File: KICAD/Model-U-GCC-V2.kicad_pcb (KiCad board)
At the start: 2 copper layers, 28.5 x 13 mm, 7 parts, among them J1 USB_C_Receptacle, J2 Conn_01x06, J3 Conn_01x02

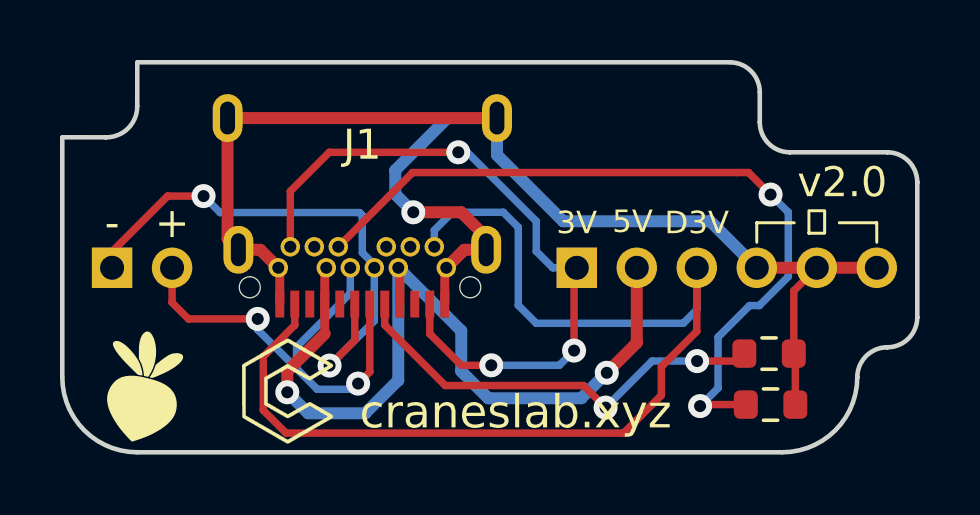
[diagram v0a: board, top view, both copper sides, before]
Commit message: 00000
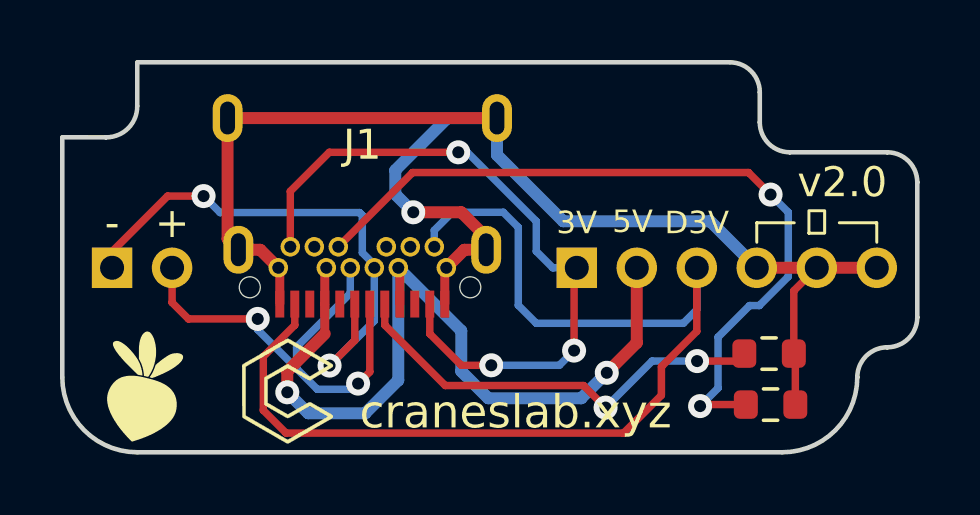
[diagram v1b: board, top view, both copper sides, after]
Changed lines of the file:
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@@
   (via (at 129.3041 107.5941) (size 0.8) (drill 0.4) (layers "F.Cu" "B.Cu") (net 5))
   (segment (start 132.65 109.75) (end 132.46 109.94) (width 0.25) (layer "B.Cu") (net 5))
-  (segment (start 130.6 108.89) (end 130.6 108.53) (width 0.25) (layer "B.Cu") (net 5))
+  (segment (start 130.6 109.25) (end 130.6 108.53) (width 0.25) (layer "B.Cu") (net 5))
   (segment (start 129.3041 107.9541) (end 129.3041 107.5941) (width 0.25) (layer "B.Cu") (net 5))
   (segment (start 132.39 106.74) (end 132.39 105.89) (width 0.25) (layer "B.Cu") (net 5))
   (segment (start 132.46 109.94) (end 131.29 109.94) (width 0.25) (layer "B.Cu") (net 5))
   (segment (start 131.29 109.94) (end 129.3041 107.9541) (width 0.25) (layer "B.Cu") (net 5))
-  (segment (start 130.6 109.25) (end 130.6 108.89) (width 0.25) (layer "B.Cu") (net 5))
   (segment (start 130.6 108.53) (end 132.39 106.74) (width 0.25) (layer "B.Cu") (net 5))
   (segment (start 126.3 103.5) (end 127.5 103.5) (width 0.25) (layer "F.Cu") (net 6))
@@
   (segment (start 137.99 107.14) (end 138.59 107.74) (width 0.25) (layer "B.Cu") (net 8))
   (segment (start 145.575 110.45) (end 144.1 110.45) (width 0.25) (layer "F.Cu") (net 9))
-  (segment (start 134.465 102.715) (end 145.265 102.715) (width 0.25) (layer "F.Cu") (net 9))
-  (segment (start 145.265 102.715) (end 145.665 102.715) (width 0.25) (layer "F.Cu") (net 9))
+  (segment (start 134.465 102.715) (end 145.665 102.715) (width 0.25) (layer "F.Cu") (net 9))
   (segment (start 131.99 105.19) (end 134.465 102.715) (width 0.25) (layer "F.Cu") (net 9))
   (segment (start 145.665 102.715) (end 146.4 103.45) (width 0.25) (layer "F.Cu") (net 9))
